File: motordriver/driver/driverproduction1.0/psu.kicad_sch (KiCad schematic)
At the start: 2 parts

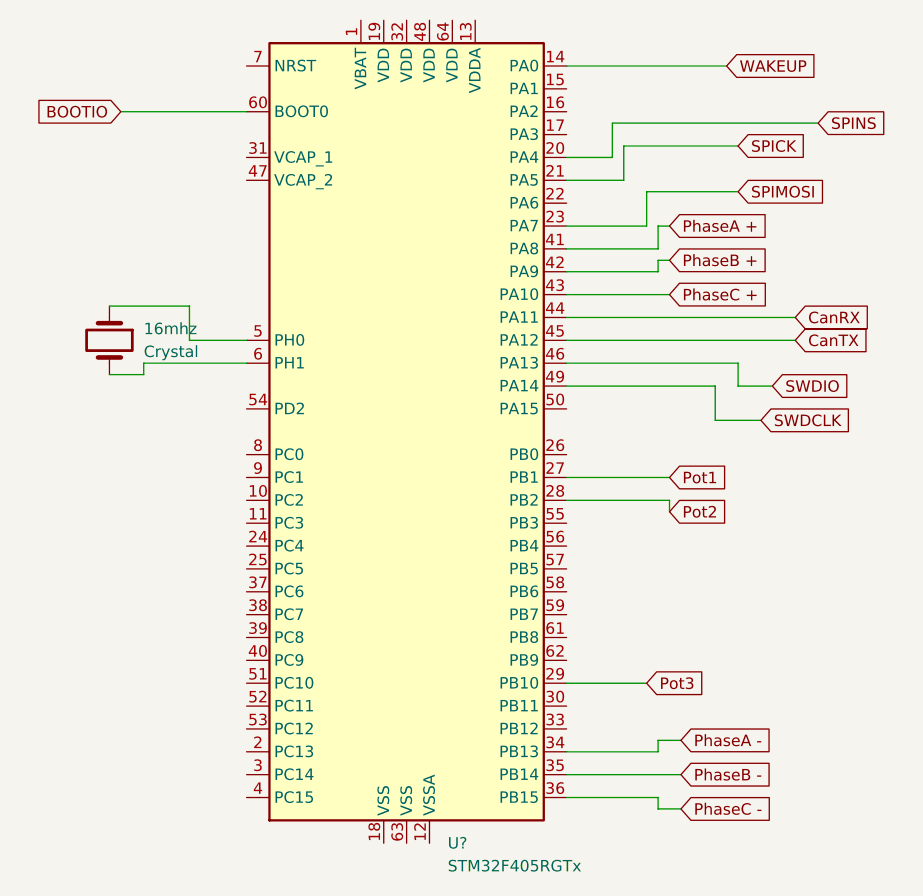
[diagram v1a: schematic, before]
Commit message: further updates
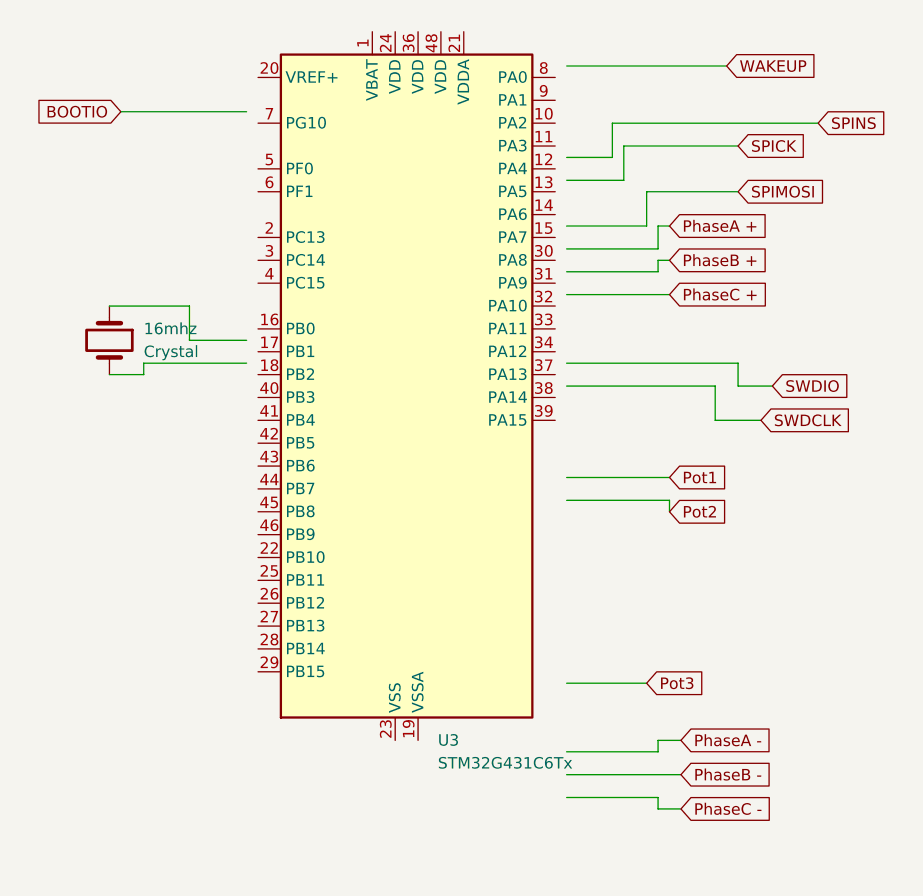
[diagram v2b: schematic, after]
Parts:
- removed U?: STM32F405RGTx, Package_QFP:LQFP-64_10x10mm_P0.5mm, symbol MCU_ST_STM32F4:STM32F405RGTx
- added U3: STM32G431C6Tx, Package_QFP:LQFP-48_7x7mm_P0.5mm, symbol MCU_ST_STM32G4:STM32G431C6Tx
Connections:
- new net: U3.23 (VSS), U3.35 (VSS), U3.47 (VSS)
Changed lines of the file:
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@@
-    (stroke (width 0) (type default))
-  )
-  (wire (pts (xy 156.21 87.63) (xy 181.61 87.63))
     (stroke (width 0) (type default))
   )
@@
   )
   (wire (pts (xy 156.21 102.87) (xy 167.64 102.87))
-    (stroke (width 0) (type default))
-  )
-  (wire (pts (xy 156.21 85.09) (xy 181.61 85.09))
     (stroke (width 0) (type default))
   )
@@
     )
   )
-  (global_label "CanRX" (shape input) (at 181.61 85.09 0) (fields_autoplaced)
-    (effects (font (size 1.27 1.27)) (justify left))
-    (property "Intersheetrefs" "${INTERSHEET_REFS}" (at 190.0707 85.0106 0)
-      (effects (font (size 1.27 1.27)) (justify left) hide)
-    )
-  )
   (global_label "PhaseB +" (shape input) (at 167.64 78.74 0) (fields_autoplaced)
     (effects (font (size 1.27 1.27)) (justify left))
@@
     (effects (font (size 1.27 1.27)) (justify left))
     (property "Intersheetrefs" "${INTERSHEET_REFS}" (at 174.4074 102.7906 0)
-      (effects (font (size 1.27 1.27)) (justify left) hide)
-    )
-  )
-  (global_label "CanTX" (shape input) (at 181.61 87.63 0) (fields_autoplaced)
-    (effects (font (size 1.27 1.27)) (justify left))
-    (property "Intersheetrefs" "${INTERSHEET_REFS}" (at 189.7683 87.5506 0)
       (effects (font (size 1.27 1.27)) (justify left) hide)
     )
@@
     )
   )
-  (symbol (lib_id "MCU_ST_STM32F4:STM32F405RGTx") (at 138.43 97.79 0) (unit 1)
+  (symbol (lib_id "MCU_ST_STM32G4:STM32G431C6Tx") (at 137.16 93.98 0) (unit 1)
     (in_bom yes) (on_board yes) (dnp no) (fields_autoplaced)
-    (property "Reference" "U?" (at 142.9894 143.51 0)
-      (effects (font (size 1.27 1.27)) (justify left))
-    )
-    (property "Value" "STM32F405RGTx" (at 142.9894 146.05 0)
-      (effects (font (size 1.27 1.27)) (justify left))
-    )
-    (property "Footprint" "Package_QFP:LQFP-64_10x10mm_P0.5mm" (at 123.19 140.97 0)
+    (property "Reference" "U3" (at 141.8941 132.08 0)
+      (effects (font (size 1.27 1.27)) (justify left))
+    )
+    (property "Value" "STM32G431C6Tx" (at 141.8941 134.62 0)
+      (effects (font (size 1.27 1.27)) (justify left))
+    )
+    (property "Footprint" "Package_QFP:LQFP-48_7x7mm_P0.5mm" (at 124.46 129.54 0)
       (effects (font (size 1.27 1.27)) (justify right) hide)
     )
-    (property "Datasheet" "http://www.st.com/st-web-ui/static/active/en/resource/technical/document/datasheet/DM00037051.pdf" (at 138.43 97.79 0)
+    (property "Datasheet" "https://www.st.com/resource/en/datasheet/stm32g431c6.pdf" (at 137.16 93.98 0)
       (effects (font (size 1.27 1.27)) hide)
     )
@@
     (pin "47")
     (pin "48")
-    (pin "49")
     (pin "5")
-    (pin "50")
-    (pin "51")
-    (pin "52")
-    (pin "53")
-    (pin "54")
-    (pin "55")
-    (pin "56")
-    (pin "57")
-    (pin "58")
-    (pin "59")
     (pin "6")
-    (pin "60")
-    (pin "61")
-    (pin "62")
-    (pin "63")
-    (pin "64")
     (pin "7")
     (pin "8")
@@
       (project "driverproduction1.0"
         (path "/80da6768-12ef-453d-855e-7545e891c31c/9b9ea144-75b3-4870-b930-183c94e89943"
-          (reference "U?") (unit 1)
+          (reference "U3") (unit 1)
         )
       )
